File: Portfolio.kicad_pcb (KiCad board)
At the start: 2 copper layers, 146 x 208 mm, 89 parts, among them J1 USB_C_Receptacle_USB2.0, SW1 SW_Push, SW2 SW_Push, SW3 SW_Push, SW4 SW_Push, U10 IS31FL3733-TQ, U11 IS31FL3733-TQ, U12 AP2112K-3.3, U13 ESP32-S3-MINI-1, U14 DS3231M, U2 NEO-M8N, U3 USR-C322, U4 BD90FC0WEFJ, U5 NEO-M8N, U6 NEO-M8N, U7 IS31FL3733-TQ, U8 IS31FL3733-TQ, U9 IS31FL3733-TQ

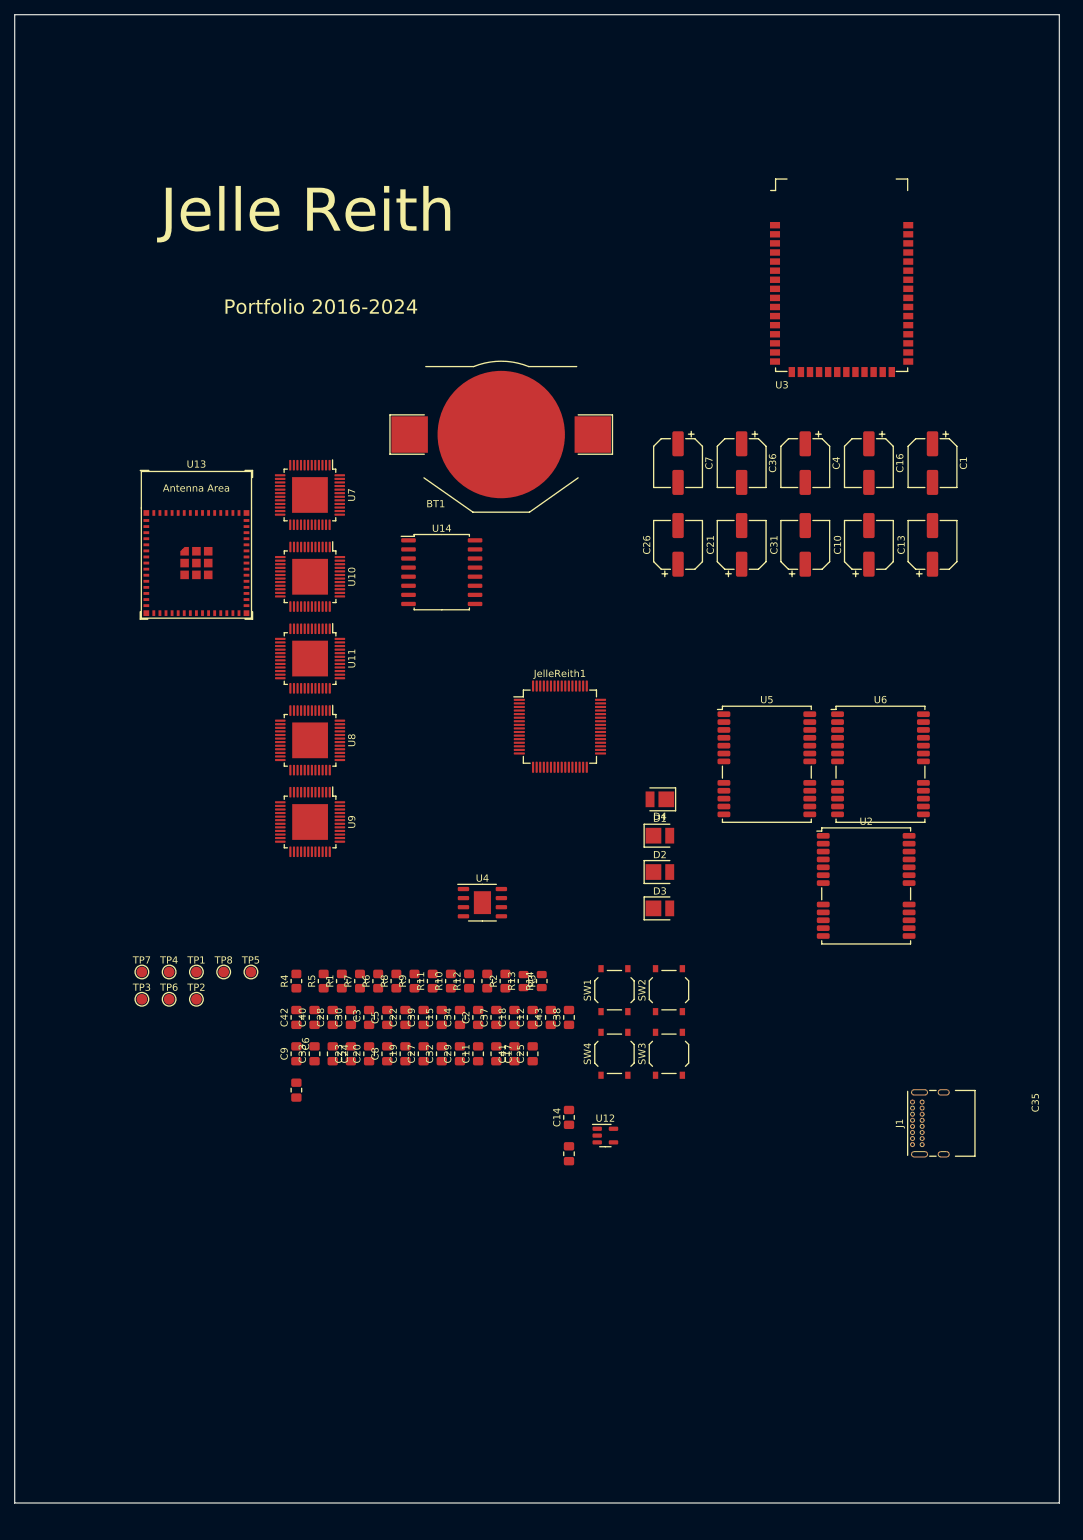
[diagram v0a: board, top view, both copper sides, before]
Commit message: >
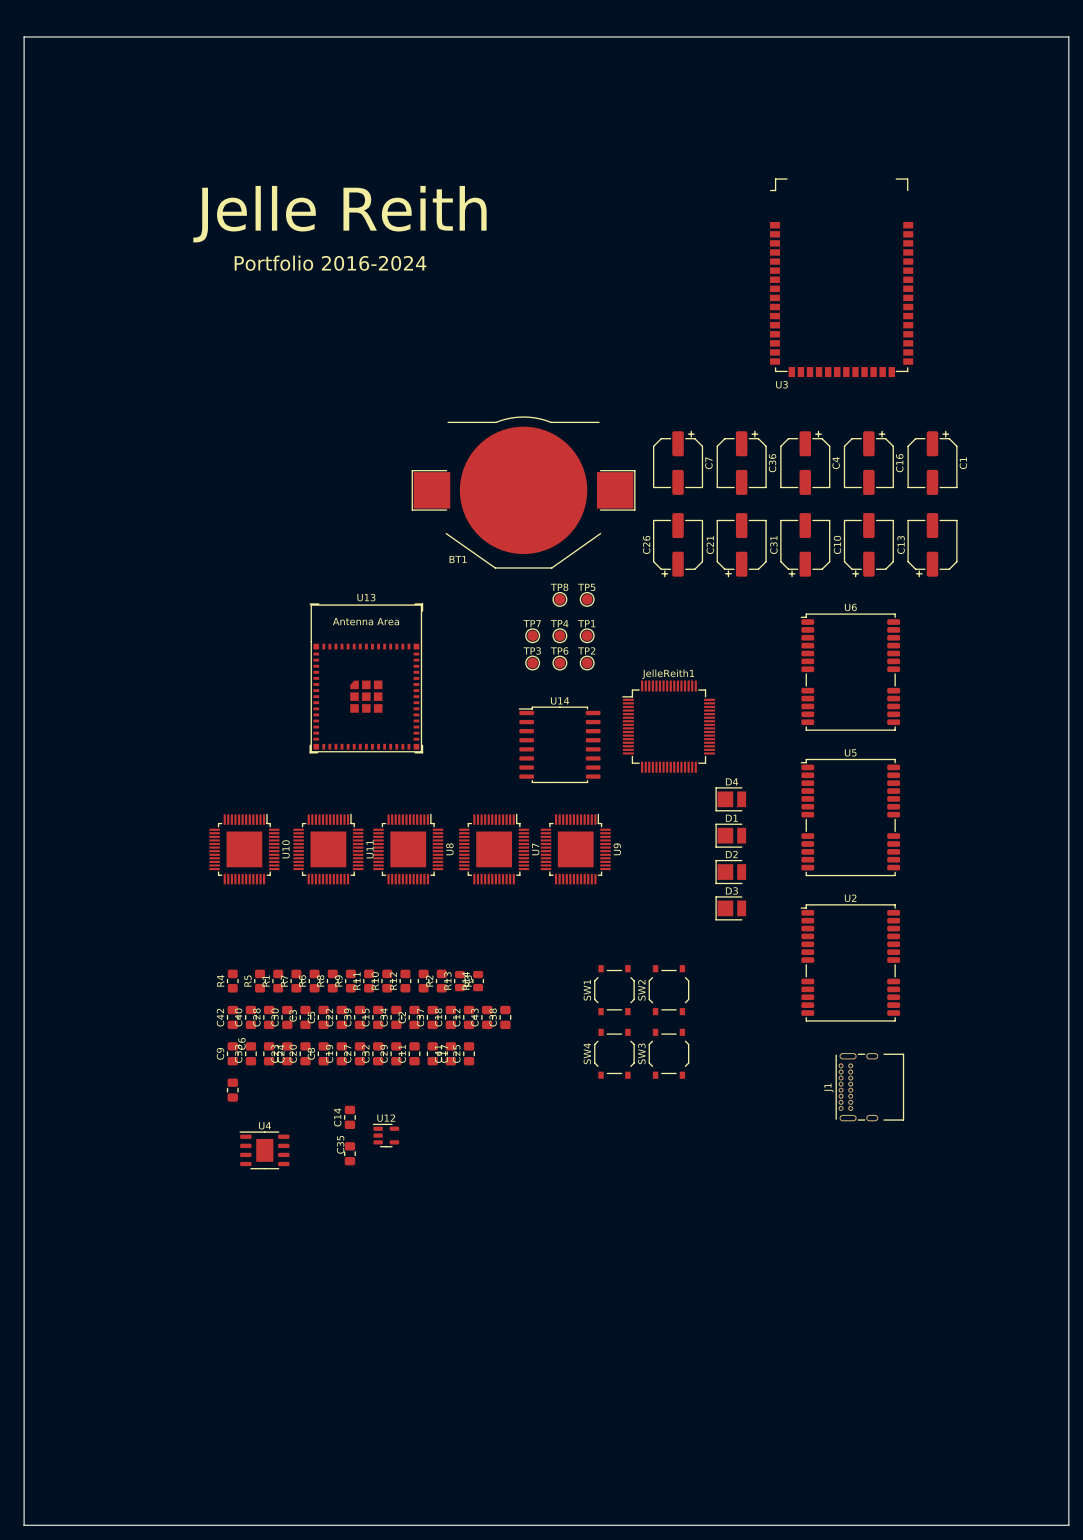
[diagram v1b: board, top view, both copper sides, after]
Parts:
- moved TP1 72.0 mm to (81.0, 87.4)
- moved TP2 72.0 mm to (81.0, 91.2)
- moved TP3 72.0 mm to (73.4, 91.2)
- moved TP4 72.0 mm to (77.2, 87.4)
- moved TP6 72.0 mm to (77.2, 91.2)
- moved TP7 72.0 mm to (73.4, 87.4)
- moved TP5 70.1 mm to (81.0, 82.3)
- moved TP8 70.1 mm to (77.2, 82.3)
- moved U7 55.8 mm to (68.0, 117.2)
- moved U4 46.1 mm to (36.0, 159.3)
- moved U10 39.2 mm to (33.1, 117.2)
- moved U9 37.3 mm to (79.4, 117.2)
- moved C14 30.6 mm to (47.9, 154.7)
- moved C35 30.6 mm to (47.9, 159.8)
- moved U12 30.6 mm to (52.9, 157.2)
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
